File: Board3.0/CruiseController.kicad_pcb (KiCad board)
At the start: 2 copper layers, 23.1 x 38 mm, 55 parts, among them J1 USB_B_Micro, J2 Conn_02x09_Top_Bottom, U1 ADG884, U3 TLV9064IRTER, U5 MIC5225, U6 MCP2562-E-MF, U7 STM32L433CCUx, Y1 32.768

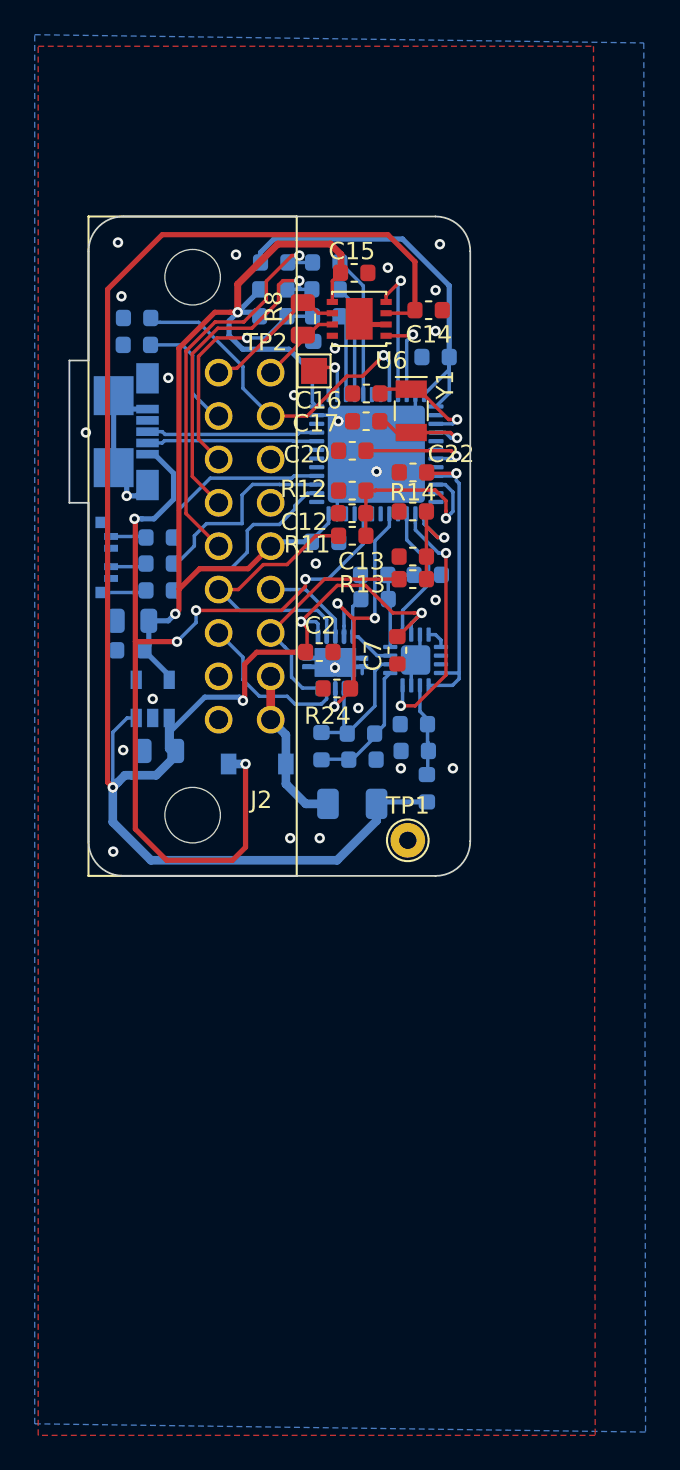
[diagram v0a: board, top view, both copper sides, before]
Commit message: Update V3
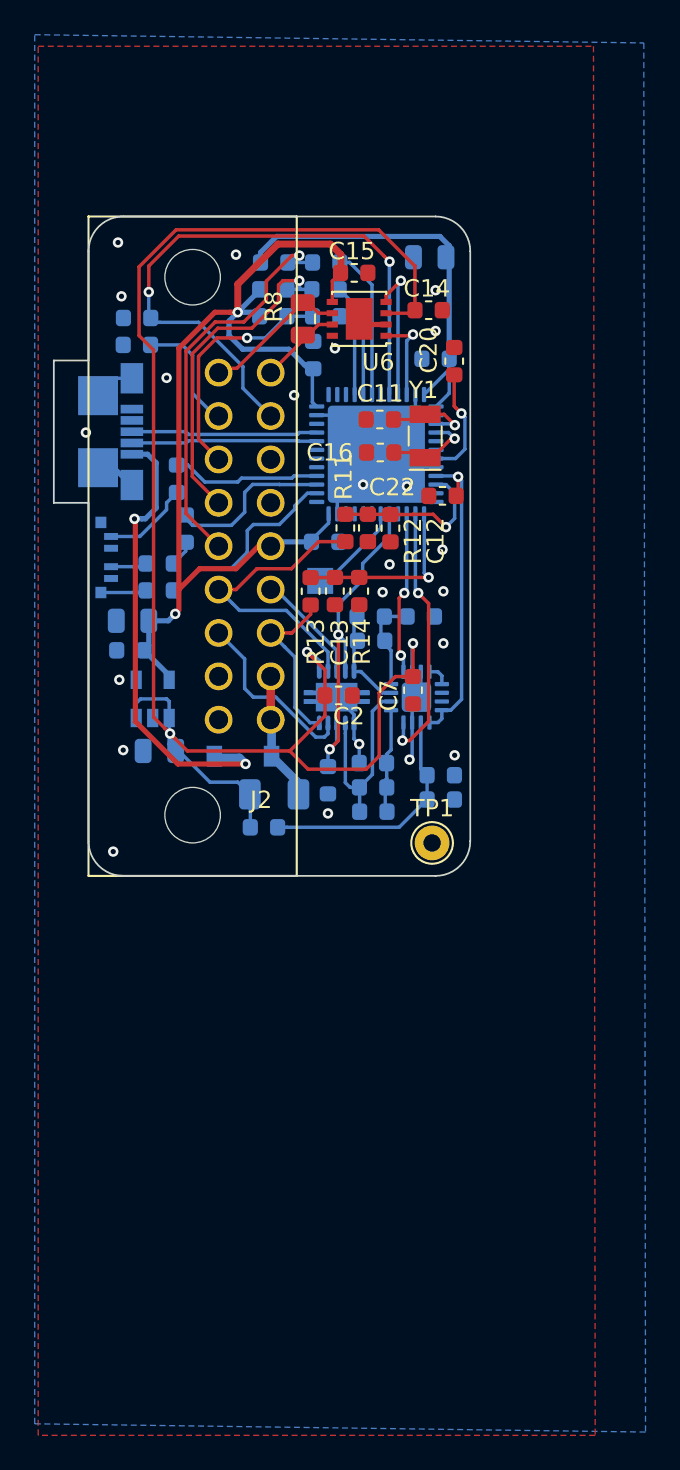
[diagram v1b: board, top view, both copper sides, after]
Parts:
- removed C17: 8pF, Capacitor_SMD:C_0603_1608Metric
- added C11: 8pF, Capacitor_SMD:C_0603_1608Metric, F.Cu at (116.8, 81.7)
- added C8: 4.7uF, Capacitor_SMD:C_0805_2012Metric, B.Cu at (119.7, 72.3)
- added R22: 50, Resistor_SMD:R_0603_1608Metric, B.Cu at (105.6, 88.0)
- R10, R9: value 27 -> 50
- R21: value 85 -> 50
- R24, TP2: moved to B.Cu
- moved TP2 12.1 mm to (113.3, 91.0)
- moved R4 9.65 mm to (110.1, 105.2), turned to 180 degrees
- moved C20 7.82 mm to (121.1, 78.3), turned to 90 degrees
- moved R13 5.93 mm to (112.8, 91.6), turned to 270 degrees
- moved R14 5.53 mm to (115.6, 91.6), turned to 90 degrees
- moved R24 5.31 mm to (113.8, 102.5), turned to 90 degrees
- moved C13 4.91 mm to (114.2, 91.6), turned to 270 degrees
- moved C5 4.81 mm to (116.4, 104.3), turned to 180 degrees
- moved C3 4.61 mm to (120.3, 103.6), turned to 0 degrees
- moved F1 4.53 mm to (110.7, 103.3), turned to 0 degrees
- moved R10 3.53 mm to (105.1, 85.1), turned to 270 degrees
- moved C16 3.49 mm to (116.8, 83.6), turned to 180 degrees
- moved R7 3.18 mm to (116.4, 102.9)
- moved C2 2.74 mm to (114.4, 97.6)
- moved C7 2.47 mm to (118.7, 97.3)
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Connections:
- C16 pad 1: GND -> Net-(C16-Pad1)
- C16 pad 2: Net-(C16-Pad2) -> GND
- R21 pad 1: LEDR -> Net-(R21-Pad1)
- U7 pad 18: Net-(U7-Pad18) -> Net-(TP2-Pad1)
- U7 pad 20: VUSB -> Net-(U7-Pad20)
- U7 pad 3: Net-(C16-Pad2) -> Net-(C11-Pad1)
- U7 pad 38: Net-(TP2-Pad1) -> Net-(U7-Pad38)
- U7 pad 39: BUTTONUP -> Net-(U7-Pad39)
- U7 pad 4: Net-(C17-Pad2) -> Net-(C16-Pad1)
- U7 pad 40: BUTTONMID -> BUTTONUP
- U7 pad 41: BUTTONDOWN -> BUTTONMID
- U7 pad 42: Net-(U7-Pad42) -> BUTTONDOWN
- Y1 pad 1: Net-(C16-Pad2) -> Net-(C16-Pad1)
- Y1 pad 2: Net-(C17-Pad2) -> Net-(C11-Pad1)
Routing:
- net VUSB: track 55.1 -> 26.6 mm, vias 5 -> 2
- net REGIN: track 115.2 -> 95.2 mm, vias 4 -> 3
- net BOOT0: track 20.2 -> 35.8 mm, vias 1 -> 2
- net Net-(C3-Pad1): track 5.27 -> 13.9 mm
- net Net-(C16-Pad2): track 6.59 -> 0.00 mm, vias 1 -> 0
- net Net-(C17-Pad2): track 6.19 -> 0.00 mm, vias 1 -> 0
- net Net-(C16-Pad1): track 0.00 -> 5.30 mm, vias 0 -> 1
- net Net-(C11-Pad1): track 0.00 -> 5.04 mm, vias 0 -> 1
- net VREFB: track 6.96 -> 10.6 mm
- net TTBIN: track 13.5 -> 9.93 mm
- net Net-(D1-Pad5): track 2.24 -> 5.09 mm
- net Net-(TP2-Pad1): track 2.90 -> 5.57 mm, vias 1 -> 0
- net Net-(C5-Pad2): track 9.53 -> 11.8 mm
- net VIN: track 10.6 -> 8.58 mm
- net VREFA: track 11.3 -> 9.56 mm
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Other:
- board size 23.1 x 38 mm -> 24 x 38 mm
